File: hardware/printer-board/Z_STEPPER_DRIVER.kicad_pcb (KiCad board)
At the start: 2 copper layers, 7 parts, among them J7 MS_SELECT, J8 TO_MOTOR, U5 A4988_MODULE

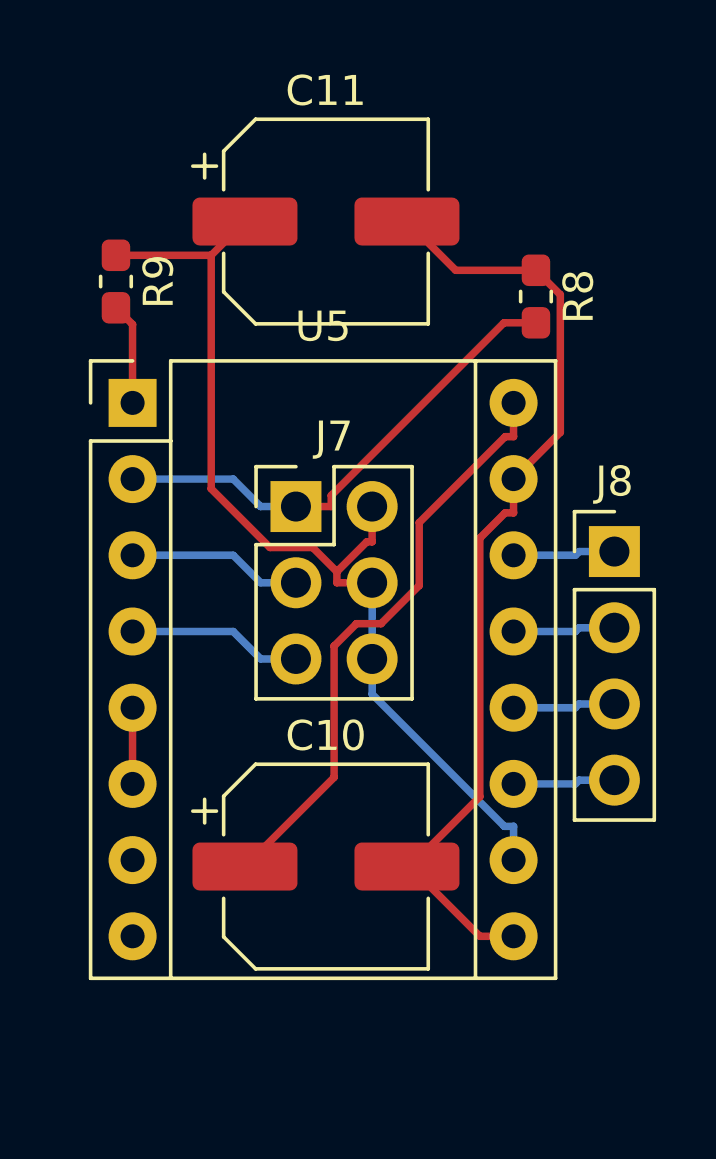
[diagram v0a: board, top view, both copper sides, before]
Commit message: update heater layouts,
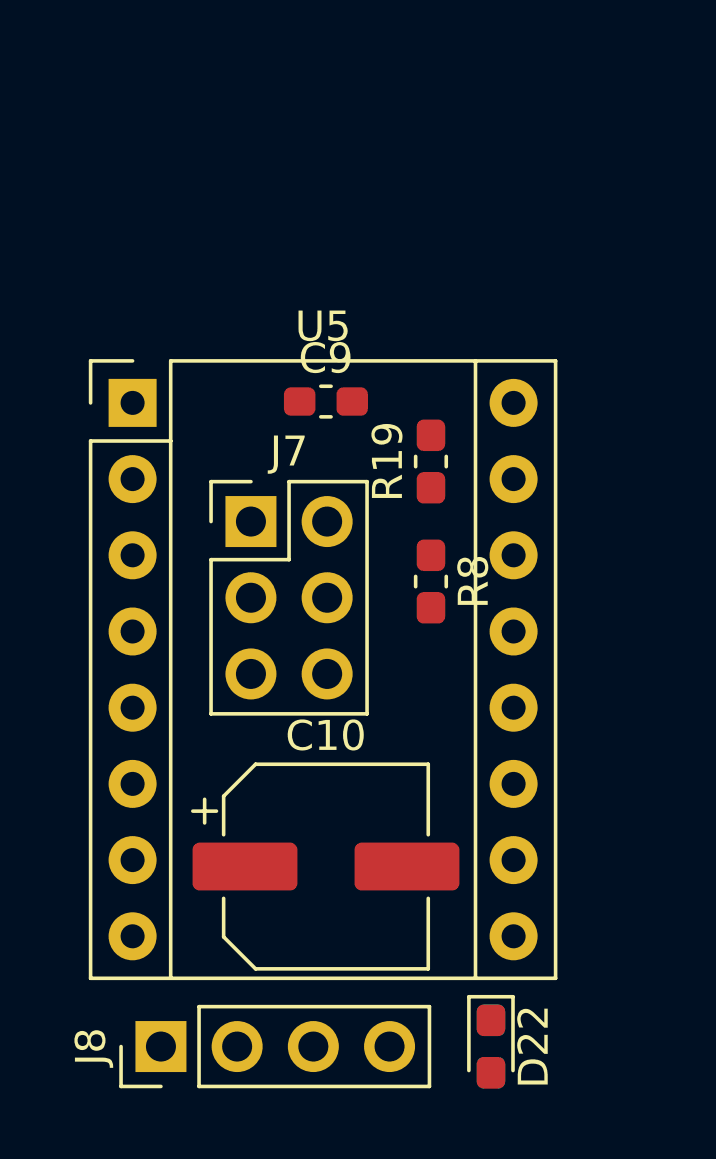
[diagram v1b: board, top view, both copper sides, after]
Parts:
- removed C11: CP100uf,25V, Capacitor_SMD:CP_Elec_6.3x7.7
- removed R9: R103,0603, Resistor_SMD:R_0603_1608Metric_Pad1.05x0.95mm_HandSolder
- added C9: C104,0603, Capacitor_SMD:C_0603_1608Metric_Pad1.05x0.95mm_HandSolder, F.Cu at (38.0, 31.5)
- added D22: LED_BLUE,0603, LED_SMD:LED_0603_1608Metric_Pad1.05x0.95mm_HandSolder, F.Cu at (43.5, 53.0)
- added R15: R102,0603, Resistor_SMD:R_0603_1608Metric_Pad1.05x0.95mm_HandSolder, B.Cu at (43.5, 53.0)
- added R19: R103,0603, Resistor_SMD:R_0603_1608Metric_Pad1.05x0.95mm_HandSolder, F.Cu at (41.5, 33.5)
- J8: value TO_MOTOR -> Z
- moved J8 22.4 mm to (32.5, 53.0), turned to 90 degrees
- moved R8 10.1 mm to (41.5, 37.5)
- moved J7 1.58 mm to (35.5, 35.5)
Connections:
- net +5V renamed +3V3_STM32
- net /DIR renamed /Z_DIR
- net /STEP renamed /Z_STEP
- U5 pad 1: /~EN~ -> /~Z_EN~
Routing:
- net +3V3_STM32: track 33.6 -> 0.00 mm
- net GND: track 31.9 -> 0.00 mm
- net +12V: track 19.8 -> 0.00 mm
- net Net-(J7-Pad1): track 16.6 -> 0.00 mm
- net Net-(J7-Pad5): track 5.82 -> 0.00 mm
- net Net-(J7-Pad3): track 5.82 -> 0.00 mm
- net Net-(J8-Pad4): track 3.41 -> 0.00 mm
- net Net-(J8-Pad3): track 3.41 -> 0.00 mm
- net Net-(J8-Pad2): track 3.41 -> 0.00 mm
- net Net-(J8-Pad1): track 3.41 -> 0.00 mm
- net /~EN~: track 3.40 -> 0.00 mm
- net Net-(U5-Pad5): track 2.54 -> 0.00 mm
